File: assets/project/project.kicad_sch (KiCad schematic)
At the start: 13 parts, among them J1 Micro SD, J2 EPD, J3 RTC, J4 Conn_01x02_Pin, SW1 SW_SPDT, U1 Reset

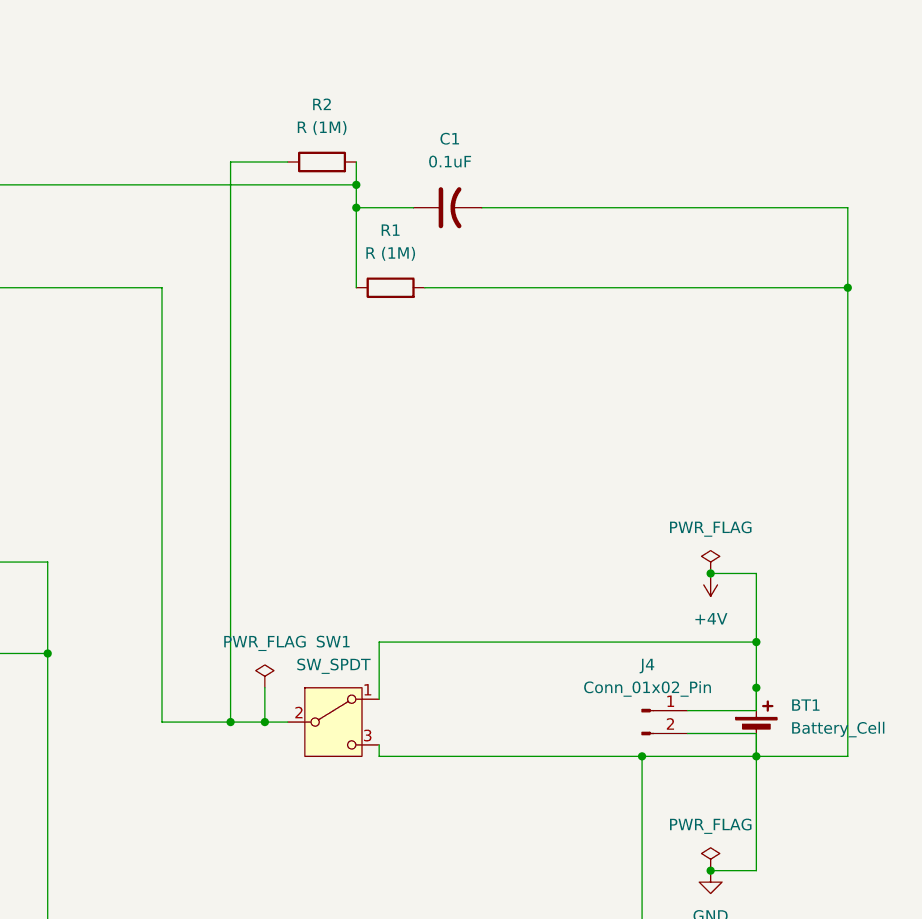
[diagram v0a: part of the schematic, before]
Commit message: kicad
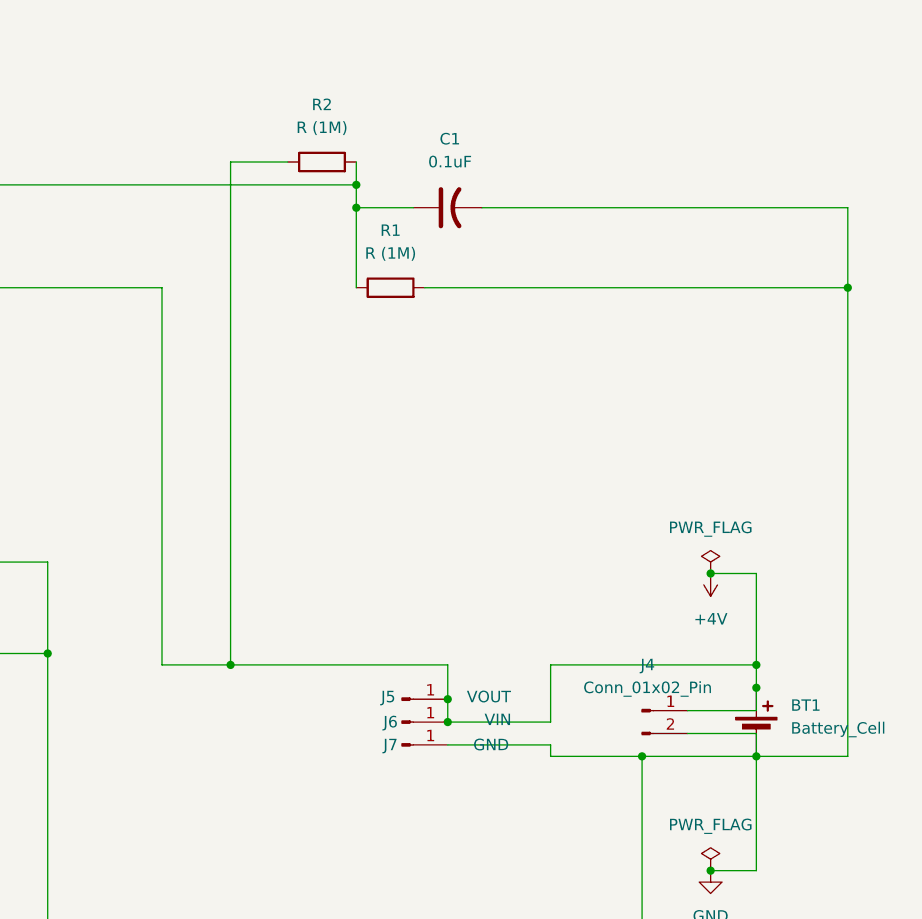
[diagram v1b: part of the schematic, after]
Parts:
- removed SW1: SW_SPDT, Button_Switch_THT:SW_Slide-03_Wuerth-WS-SLTV_10x2.5x6.4_P2.54mm, symbol Switch:SW_SPDT
- added J5: VOUT, Connector_Pin:Pin_D1.3mm_L10.0mm_W3.5mm_Flat, symbol Connector:Conn_01x01_Pin
- added J6: VIN, Connector_Pin:Pin_D1.3mm_L10.0mm_W3.5mm_Flat, symbol Connector:Conn_01x01_Pin
- added J7: GND, Connector_Pin:Pin_D1.3mm_L10.0mm_W3.5mm_Flat, symbol Connector:Conn_01x01_Pin
- U1: footprint Button_Switch_THT:SW_Push_2P1T_Toggle_CK_PVA1xxH1xxxxxxV2 -> Button_Switch_THT:SW_PUSH_6mm
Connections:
- net +4V: now also A1.30 (VIN), R2.1, J5.1 (Pin_1), J6.1 (Pin_1)
- net GND: now also J7.1 (Pin_1)
